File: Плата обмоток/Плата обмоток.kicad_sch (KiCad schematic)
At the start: 14 parts, among them J1 4900, J10 4900, J11 4900, J12 4900, J13 4900, J2 4900, J3 4900, J4 Conn_01x02, J6 Conn_01x02, J7 Conn_01x02, J8 4900, J8 Conn_02x02_Odd_Even, J9 4900

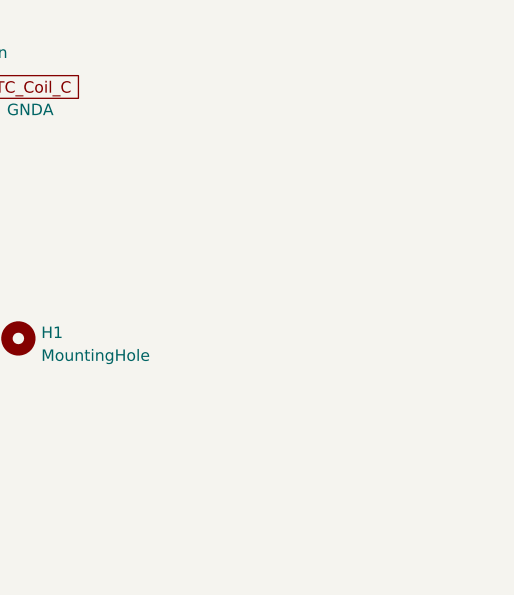
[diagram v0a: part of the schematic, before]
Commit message: Расставил ножевые разъёмы финально
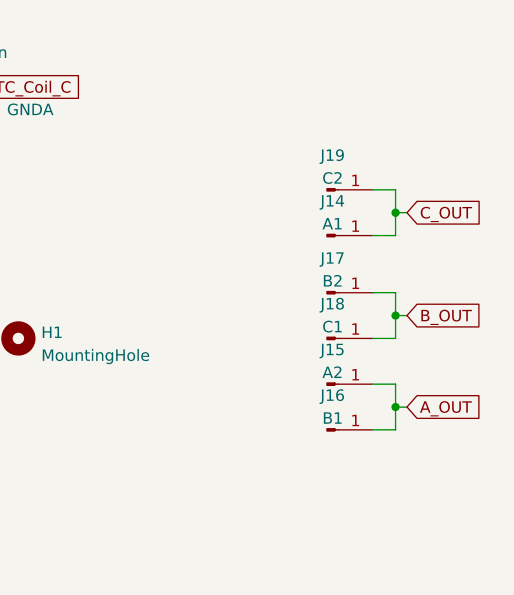
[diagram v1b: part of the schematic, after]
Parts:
- added J14: A1, Connector_My:Coil, symbol Connector:Conn_01x01_Pin
- added J15: A2, Connector_My:Coil, symbol Connector:Conn_01x01_Pin
- added J16: B1, Connector_My:Coil, symbol Connector:Conn_01x01_Pin
- added J17: B2, Connector_My:Coil, symbol Connector:Conn_01x01_Pin
- added J18: C1, Connector_My:Coil, symbol Connector:Conn_01x01_Pin
- added J19: C2, Connector_My:Coil, symbol Connector:Conn_01x01_Pin
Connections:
- net A_OUT: now also J15.1 (Pin_1), J16.1 (Pin_1)
- net B_OUT: now also J17.1 (Pin_1), J18.1 (Pin_1)
- net C_OUT: now also J14.1 (Pin_1), J19.1 (Pin_1)
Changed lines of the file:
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@@
   (junction (at 99.06 123.19) (diameter 0) (color 0 0 0 0)
   )
+  (junction (at 234.95 80.01) (diameter 0) (color 0 0 0 0)
+  )
+  (junction (at 234.95 58.42) (diameter 0) (color 0 0 0 0)
+  )
   (junction (at 64.77 116.84) (diameter 0) (color 0 0 0 0)
   )
@@
   (junction (at 99.06 116.84) (diameter 0) (color 0 0 0 0)
   )
+  (junction (at 234.95 69.85) (diameter 0) (color 0 0 0 0)
+  )
   (junction (at 64.77 114.3) (diameter 0) (color 0 0 0 0)
   )
@@
     (stroke (width 0) (type default))
   )
+  (wire (pts (xy 232.41 82.55) (xy 234.95 82.55))
+    (stroke (width 0) (type default))
+  )
   (wire (pts (xy 66.04 105.41) (xy 64.77 105.41))
     (stroke (width 0) (type default))
   )
+  (wire (pts (xy 234.95 55.88) (xy 234.95 58.42))
+    (stroke (width 0) (type default))
+  )
   (wire (pts (xy 133.35 107.95) (xy 134.62 107.95))
     (stroke (width 0) (type default))
   )
+  (wire (pts (xy 234.95 80.01) (xy 234.95 77.47))
+    (stroke (width 0) (type default))
+  )
   (wire (pts (xy 64.77 123.19) (xy 64.77 125.73))
     (stroke (width 0) (type default))
@@
     (stroke (width 0) (type default))
   )
+  (wire (pts (xy 232.41 67.31) (xy 234.95 67.31))
+    (stroke (width 0) (type default))
+  )
+  (wire (pts (xy 234.95 67.31) (xy 234.95 69.85))
+    (stroke (width 0) (type default))
+  )
+  (wire (pts (xy 234.95 77.47) (xy 232.41 77.47))
+    (stroke (width 0) (type default))
+  )
   (wire (pts (xy 99.06 114.3) (xy 100.33 114.3))
     (stroke (width 0) (type default))
@@
     (stroke (width 0) (type default))
   )
+  (wire (pts (xy 234.95 69.85) (xy 234.95 72.39))
+    (stroke (width 0) (type default))
+  )
   (wire (pts (xy 64.77 116.84) (xy 66.04 116.84))
     (stroke (width 0) (type default))
@@
     (stroke (width 0) (type default))
   )
+  (wire (pts (xy 234.95 58.42) (xy 236.22 58.42))
+    (stroke (width 0) (type default))
+  )
   (wire (pts (xy 133.35 123.19) (xy 133.35 125.73))
     (stroke (width 0) (type default))
@@
     (stroke (width 0) (type default))
   )
+  (wire (pts (xy 232.41 55.88) (xy 234.95 55.88))
+    (stroke (width 0) (type default))
+  )
+  (wire (pts (xy 234.95 69.85) (xy 236.22 69.85))
+    (stroke (width 0) (type default))
+  )
   (wire (pts (xy 64.77 125.73) (xy 66.04 125.73))
     (stroke (width 0) (type default))
@@
     (stroke (width 0) (type default))
   )
+  (wire (pts (xy 234.95 82.55) (xy 234.95 80.01))
+    (stroke (width 0) (type default))
+  )
   (wire (pts (xy 99.06 123.19) (xy 100.33 123.19))
     (stroke (width 0) (type default))
   )
+  (wire (pts (xy 232.41 60.96) (xy 234.95 60.96))
+    (stroke (width 0) (type default))
+  )
+  (wire (pts (xy 234.95 80.01) (xy 236.22 80.01))
+    (stroke (width 0) (type default))
+  )
   (wire (pts (xy 64.77 107.95) (xy 64.77 114.3))
     (stroke (width 0) (type default))
@@
   )
   (wire (pts (xy 64.77 105.41) (xy 64.77 107.95))
+    (stroke (width 0) (type default))
+  )
+  (wire (pts (xy 234.95 72.39) (xy 232.41 72.39))
+    (stroke (width 0) (type default))
+  )
+  (wire (pts (xy 234.95 58.42) (xy 234.95 60.96))
     (stroke (width 0) (type default))
   )
@@
     )
   )
+  (global_label "C_OUT" (shape input) (at 236.22 58.42 0) (fields_autoplaced)
+    (effects (font (size 1.27 1.27)) (justify left))
+    (property "Intersheetrefs" "${INTERSHEET_REFS}" (at 244.992 58.42 0)
+      (effects (font (size 1.27 1.27)) (justify left) hide)
+    )
+  )
   (global_label "PTC_Coil_C" (shape input) (at 140.97 85.09 180) (fields_autoplaced)
     (effects (font (size 1.27 1.27)) (justify right))
@@
     )
   )
+  (global_label "A_OUT" (shape input) (at 236.22 80.01 0) (fields_autoplaced)
+    (effects (font (size 1.27 1.27)) (justify left))
+    (property "Intersheetrefs" "${INTERSHEET_REFS}" (at 244.8106 80.01 0)
+      (effects (font (size 1.27 1.27)) (justify left) hide)
+    )
+  )
   (global_label "A_OUT" (shape input) (at 62.23 115.57 180) (fields_autoplaced)
     (effects (font (size 1.27 1.27)) (justify right))
@@
     )
   )
+  (global_label "B_OUT" (shape input) (at 236.22 69.85 0) (fields_autoplaced)
+    (effects (font (size 1.27 1.27)) (justify left))
+    (property "Intersheetrefs" "${INTERSHEET_REFS}" (at 244.992 69.85 0)
+      (effects (font (size 1.27 1.27)) (justify left) hide)
+    )
+  )
+  (symbol (lib_id "Connector:Conn_01x01_Pin") (at 227.33 60.96 0) (unit 1)
+    (in_bom yes) (on_board yes) (dnp no) (fields_autoplaced)
+    (property "Reference" "J14" (at 227.965 57.15 0)
+      (effects (font (size 1.27 1.27)))
+    )
+    (property "Value" "A1" (at 227.965 59.69 0)
+      (effects (font (size 1.27 1.27)))
+    )
+    (property "Footprint" "Connector_My:Coil" (at 227.33 60.96 0)
+      (effects (font (size 1.27 1.27)) hide)
+    )
+    (property "Datasheet" "~" (at 227.33 60.96 0)
+      (effects (font (size 1.27 1.27)) hide)
+    )
+    (pin "1")
+    (instances
+      (project "Плата обмоток"
+        (path "/7abc0ce6-258d-434e-9c1a-83bc5738d31c"
+          (reference "J14") (unit 1)
+        )
+      )
+    )
+  )
   (symbol (lib_id "4900:4900") (at 134.62 105.41 0) (unit 1)
     (in_bom yes) (on_board yes) (dnp no) (fields_autoplaced)
@@
         (path "/7abc0ce6-258d-434e-9c1a-83bc5738d31c"
           (reference "J11") (unit 1)
+        )
+      )
+    )
+  )
+  (symbol (lib_id "Connector:Conn_01x01_Pin") (at 227.33 72.39 0) (unit 1)
+    (in_bom yes) (on_board yes) (dnp no) (fields_autoplaced)
+    (property "Reference" "J18" (at 227.965 68.58 0)
+      (effects (font (size 1.27 1.27)))
+    )
+    (property "Value" "C1" (at 227.965 71.12 0)
+      (effects (font (size 1.27 1.27)))
+    )
+    (property "Footprint" "Connector_My:Coil" (at 227.33 72.39 0)
+      (effects (font (size 1.27 1.27)) hide)
+    )
+    (property "Datasheet" "~" (at 227.33 72.39 0)
+      (effects (font (size 1.27 1.27)) hide)
+    )
+    (pin "1")
+    (instances
+      (project "Плата обмоток"
+        (path "/7abc0ce6-258d-434e-9c1a-83bc5738d31c"
+          (reference "J18") (unit 1)
         )
       )
@@
     )
   )
+  (symbol (lib_id "Connector:Conn_01x01_Pin") (at 227.33 77.47 0) (unit 1)
+    (in_bom yes) (on_board yes) (dnp no) (fields_autoplaced)
+    (property "Reference" "J15" (at 227.965 73.66 0)
+      (effects (font (size 1.27 1.27)))
+    )
+    (property "Value" "A2" (at 227.965 76.2 0)
+      (effects (font (size 1.27 1.27)))
+    )
+    (property "Footprint" "Connector_My:Coil" (at 227.33 77.47 0)
+      (effects (font (size 1.27 1.27)) hide)
+    )
+    (property "Datasheet" "~" (at 227.33 77.47 0)
+      (effects (font (size 1.27 1.27)) hide)
+    )
+    (pin "1")
+    (instances
+      (project "Плата обмоток"
+        (path "/7abc0ce6-258d-434e-9c1a-83bc5738d31c"
+          (reference "J15") (unit 1)
+        )
+      )
+    )
+  )
   (symbol (lib_id "4900:4900") (at 66.04 105.41 0) (unit 1)
     (in_bom yes) (on_board yes) (dnp no) (fields_autoplaced)
@@
         (path "/7abc0ce6-258d-434e-9c1a-83bc5738d31c"
           (reference "J1") (unit 1)
+        )
+      )
+    )
+  )
+  (symbol (lib_id "Connector:Conn_01x01_Pin") (at 227.33 67.31 0) (unit 1)
+    (in_bom yes) (on_board yes) (dnp no) (fields_autoplaced)
+    (property "Reference" "J17" (at 227.965 63.5 0)
+      (effects (font (size 1.27 1.27)))
+    )
+    (property "Value" "B2" (at 227.965 66.04 0)
+      (effects (font (size 1.27 1.27)))
+    )
+    (property "Footprint" "Connector_My:Coil" (at 227.33 67.31 0)
+      (effects (font (size 1.27 1.27)) hide)
+    )
+    (property "Datasheet" "~" (at 227.33 67.31 0)
+      (effects (font (size 1.27 1.27)) hide)
+    )
+    (pin "1")
+    (instances
+      (project "Плата обмоток"
+        (path "/7abc0ce6-258d-434e-9c1a-83bc5738d31c"
+          (reference "J17") (unit 1)
         )
       )
@@
     )
   )
+  (symbol (lib_id "Connector:Conn_01x01_Pin") (at 227.33 55.88 0) (unit 1)
+    (in_bom yes) (on_board yes) (dnp no)
+    (property "Reference" "J19" (at 227.965 52.07 0)
+      (effects (font (size 1.27 1.27)))
+    )
+    (property "Value" "C2" (at 227.965 54.61 0)
+      (effects (font (size 1.27 1.27)))
+    )
+    (property "Footprint" "Connector_My:Coil" (at 227.33 55.88 0)
+      (effects (font (size 1.27 1.27)) hide)
+    )
+    (property "Datasheet" "~" (at 227.33 55.88 0)
+      (effects (font (size 1.27 1.27)) hide)
+    )
+    (pin "1")
+    (instances
+      (project "Плата обмоток"
+        (path "/7abc0ce6-258d-434e-9c1a-83bc5738d31c"
+          (reference "J19") (unit 1)
+        )
+      )
+    )
+  )
   (symbol (lib_id "4900:4900") (at 66.04 123.19 0) (unit 1)
     (in_bom yes) (on_board yes) (dnp no) (fields_autoplaced)
@@
         )
       )
+    )
+  )
+  (symbol (lib_id "Connector:Conn_01x01_Pin") (at 227.33 82.55 0) (unit 1)
+    (in_bom yes) (on_board yes) (dnp no) (fields_autoplaced)
+    (property "Reference" "J16" (at 227.965 78.74 0)
+      (effects (font (size 1.27 1.27)))
+    )
+    (property "Value" "B1" (at 227.965 81.28 0)
+      (effects (font (size 1.27 1.27)))
+    )
+    (property "Footprint" "Connector_My:Coil" (at 227.33 82.55 0)
+      (effects (font (size 1.27 1.27)) hide)
+    )
+    (property "Datasheet" "~" (at 227.33 82.55 0)
+      (effects (font (size 1.27 1.27)) hide)
+    )
+    (pin "1")
+    (instances
+      (project "Плата обмоток"
+        (path "/7abc0ce6-258d-434e-9c1a-83bc5738d31c"
+          (reference "J16") (unit 1)
+        )
+      )
